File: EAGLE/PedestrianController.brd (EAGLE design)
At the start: 30 x 80 mm, 16 parts, among them CON1 FTDI, CON2 DS3231, CON3 AC110V, CON4 SIGNAL, IC1 ESP-WROOM-02

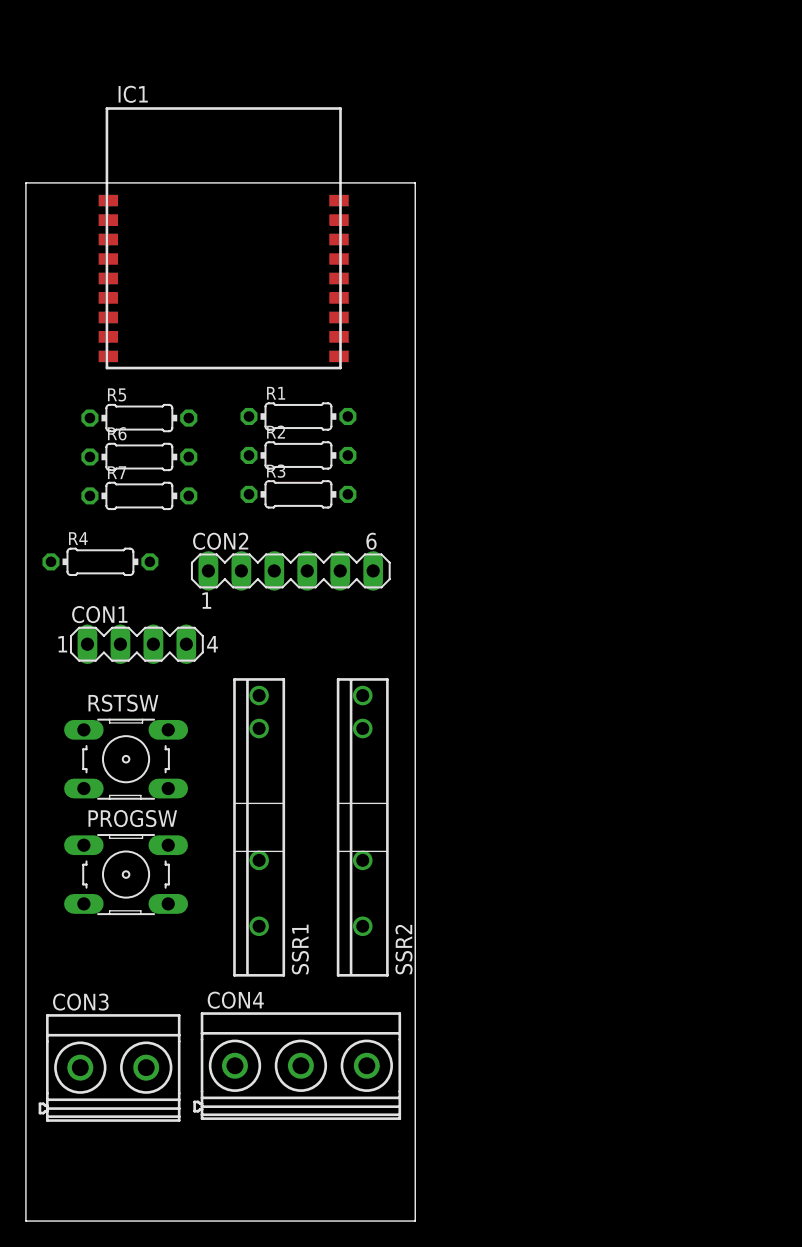
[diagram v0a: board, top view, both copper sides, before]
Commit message: Rearranged.
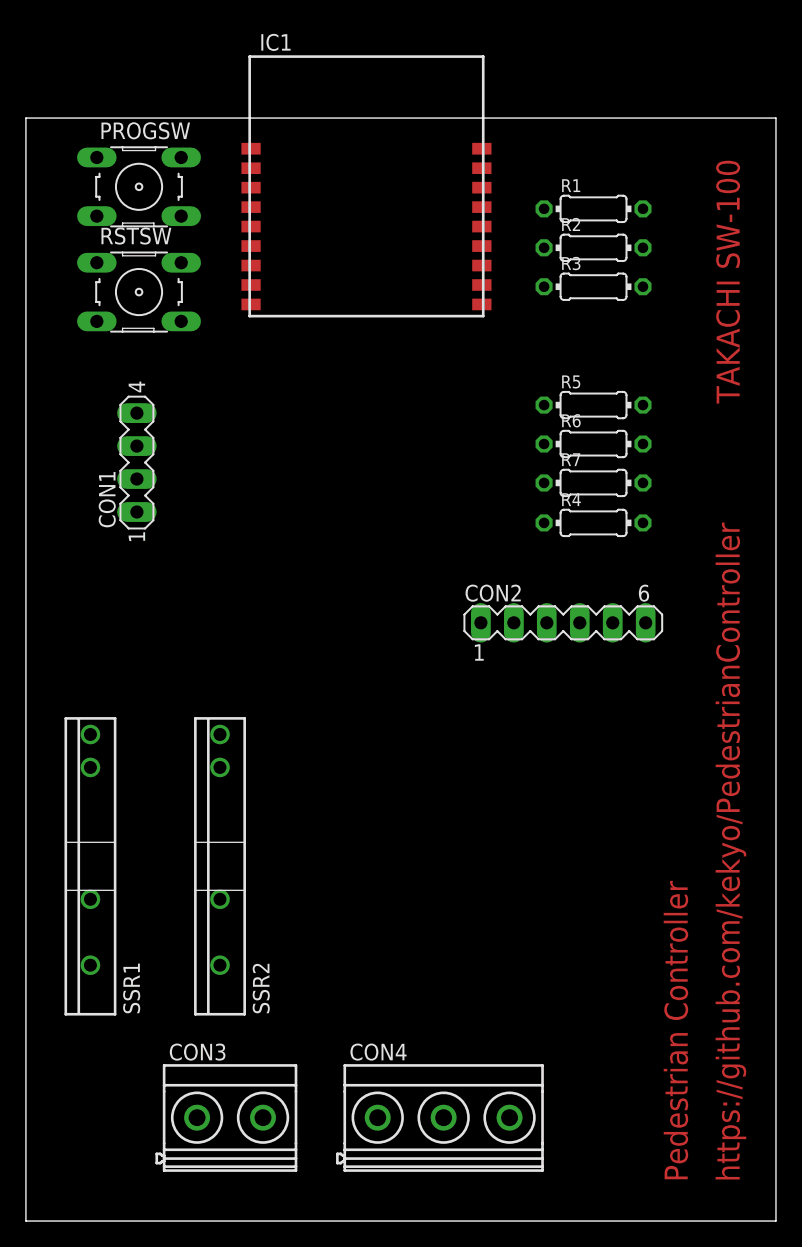
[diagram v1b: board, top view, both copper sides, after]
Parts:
- moved PROGSW 53.0 mm to (8.71, 79.7)
- moved R4 38.1 mm to (43.7, 53.8)
- moved RSTSW 36.0 mm to (8.71, 71.6)
- moved R5 35.0 mm to (43.7, 62.9)
- moved R6 35.0 mm to (43.7, 59.9)
- moved R7 35.0 mm to (43.7, 56.9)
- moved R1 27.8 mm to (43.7, 78.0)
- moved R2 27.8 mm to (43.7, 75.0)
- moved R3 27.8 mm to (43.7, 72.0)
- moved CON2 21.4 mm to (41.4, 46.1)
- moved CON1 14.0 mm to (8.55, 58.5), turned to 90 degrees
- moved SSR1 13.3 mm to (4.97, 27.3)
- moved CON4 11.7 mm to (34.8, 7.94)
- moved IC1 11.7 mm to (26.2, 77.7)
- moved SSR2 11.4 mm to (15.0, 27.3)
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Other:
- board size 30 x 80 mm -> 57.8 x 85 mm
- board text added: "Pedestrian Controller"
- board text added: "TAKACHI SW-100"
- board text added: "https://github.com/kekyo/PedestrianController"
